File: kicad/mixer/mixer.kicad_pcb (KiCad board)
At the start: 2 copper layers, 100 x 100 mm, 83 parts, among them J1 RETURN_L, J10 CH4_IN, J11 CH5_IN, J12 EURO_PWR_2x5, J2 RETURN_R, J3 SEND_L, J4 SEND_R, J5 MIX_L, J6 MIX_R, J7 CH1_IN, J8 CH2_IN, J9 CH3_IN, U1 TL074, U2 TL074

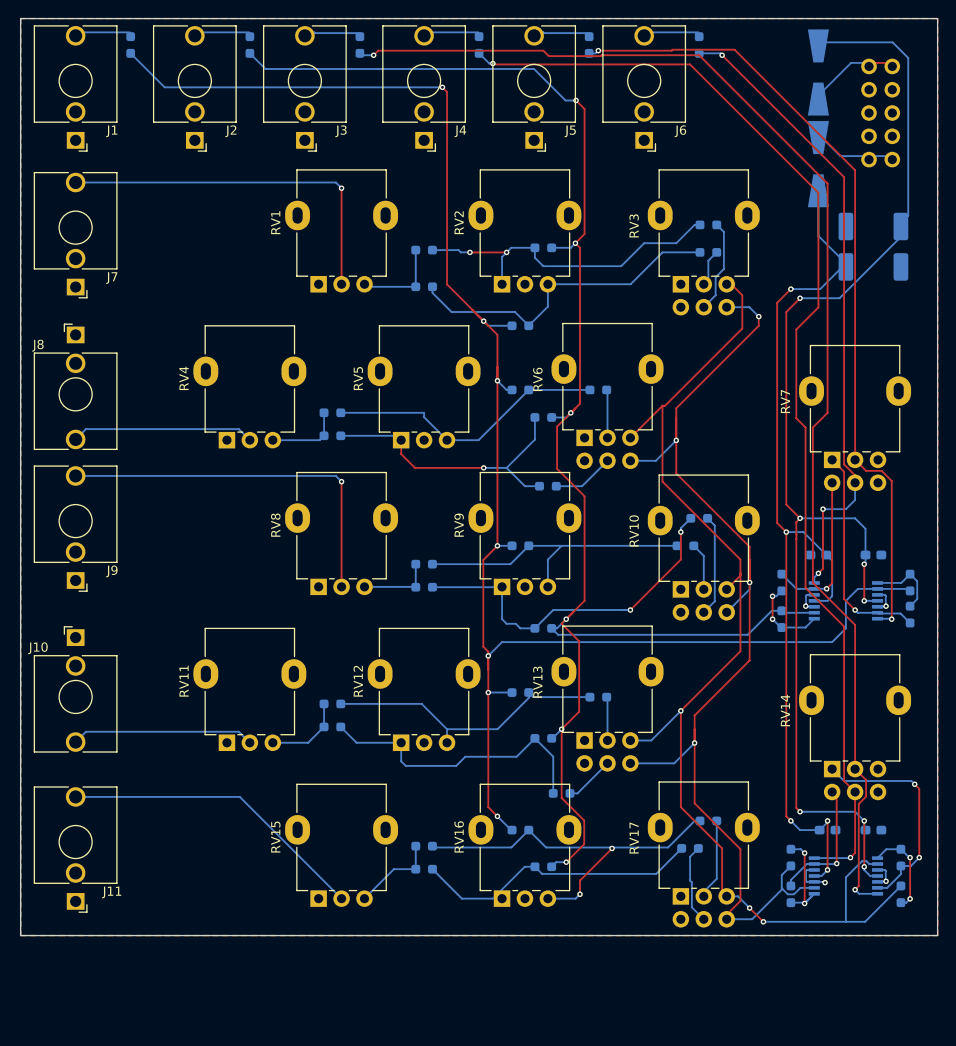
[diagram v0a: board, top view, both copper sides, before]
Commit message: been a minute huh
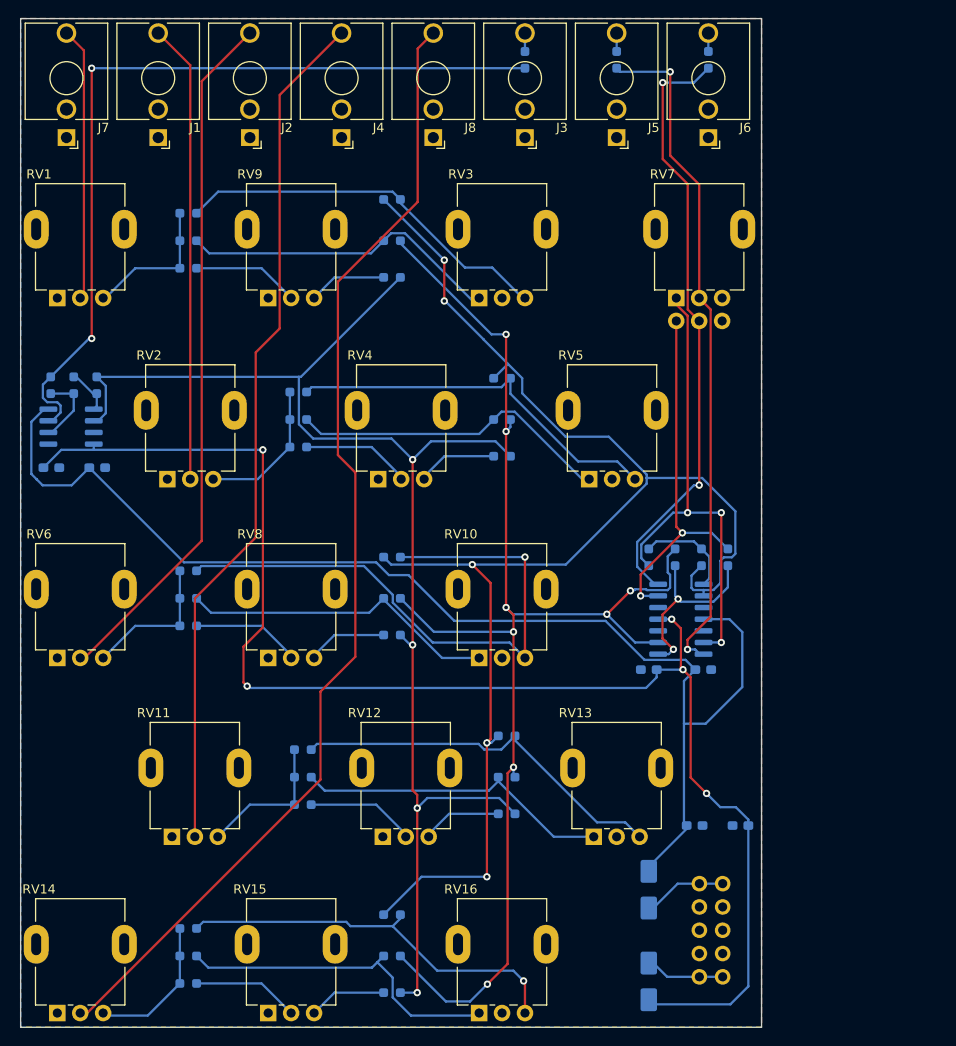
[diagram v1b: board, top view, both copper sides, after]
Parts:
- removed J10: CH4_IN, Connector_Audio:Jack_3.5mm_QingPu_WQP-PJ398SM_Vertical_CircularHoles
- removed J11: CH5_IN, Connector_Audio:Jack_3.5mm_QingPu_WQP-PJ398SM_Vertical_CircularHoles
- removed J9: CH3_IN, Connector_Audio:Jack_3.5mm_QingPu_WQP-PJ398SM_Vertical_CircularHoles
- removed R40, R41: 100k, Resistor_SMD:R_0603_1608Metric_Pad0.98x0.95mm_HandSolder
- removed R42: 10k, Resistor_SMD:R_0603_1608Metric_Pad0.98x0.95mm_HandSolder
- removed R44: 4k7, Resistor_SMD:R_0603_1608Metric_Pad0.98x0.95mm_HandSolder
- removed RV17: A10k, Potentiometer_THT:Potentiometer_Alpha_RD902F-40-00D_Dual_Vertical
- added REF**: LOGO, KitsBlips:logo, B.Cu at (142.0, 56.0)
- C1, C2: footprint Capacitor_SMD:CP_Elec_5x5.3 -> Capacitor_SMD:C_0603_1608Metric_Pad1.08x0.95mm_HandSolder
- D1, D2: value B140-E3/61T -> SS14; footprint Diode_SMD:D_SMA-SMB_Universal_Handsoldering -> Diode_SMD:D_SMA
- J1: value RETURN_L -> MONO_IN; footprint Connector_Audio:Jack_3.5mm_QingPu_WQP-PJ398SM_Vertical_CircularHoles -> KitsBlips:Jack_3.5mm_QingPu_WQP-PJ398SM_Vertical_CircularHoles
- J2: value RETURN_R -> MONO_IN; footprint Connector_Audio:Jack_3.5mm_QingPu_WQP-PJ398SM_Vertical_CircularHoles -> KitsBlips:Jack_3.5mm_QingPu_WQP-PJ398SM_Vertical_CircularHoles
- J3, J5, J6: footprint Connector_Audio:Jack_3.5mm_QingPu_WQP-PJ398SM_Vertical_CircularHoles -> KitsBlips:Jack_3.5mm_QingPu_WQP-PJ398SM_Vertical_CircularHoles
- J4: value SEND_R -> MONO_IN; footprint Connector_Audio:Jack_3.5mm_QingPu_WQP-PJ398SM_Vertical_CircularHoles -> KitsBlips:Jack_3.5mm_QingPu_WQP-PJ398SM_Vertical_CircularHoles
- J7: value CH1_IN -> MONO_IN; footprint Connector_Audio:Jack_3.5mm_QingPu_WQP-PJ398SM_Vertical_CircularHoles -> KitsBlips:Jack_3.5mm_QingPu_WQP-PJ398SM_Vertical_CircularHoles
- J8: value CH2_IN -> MONO_IN; footprint Connector_Audio:Jack_3.5mm_QingPu_WQP-PJ398SM_Vertical_CircularHoles -> KitsBlips:Jack_3.5mm_QingPu_WQP-PJ398SM_Vertical_CircularHoles
- R10, R11, R22, R31, R32, R38: value 10k -> 100k
- R13, R19, R25, R29, R33, R34, R35, R5, R6, R7, R8, R9: value 100k -> 10k
- R3: value 1k -> 10k
- R39: value 4k7 -> 10k
- RV1, RV11, RV15, RV16, RV4, RV5, RV8: footprint Potentiometer_THT:Potentiometer_Alpha_RD901F-40-00D_Single_Vertical -> KitsBlips:Potentiometer_Alpha_RD901F-40-00D_Single_Vertical
- RV10, RV13, RV3: value A10k -> B10k; footprint Potentiometer_THT:Potentiometer_Alpha_RD902F-40-00D_Dual_Vertical -> KitsBlips:Potentiometer_Alpha_RD901F-40-00D_Single_Vertical
- RV12, RV2, RV9: value B10k -> A10k; footprint Potentiometer_THT:Potentiometer_Alpha_RD901F-40-00D_Single_Vertical -> KitsBlips:Potentiometer_Alpha_RD901F-40-00D_Single_Vertical
- RV14, RV6: footprint Potentiometer_THT:Potentiometer_Alpha_RD902F-40-00D_Dual_Vertical -> KitsBlips:Potentiometer_Alpha_RD901F-40-00D_Single_Vertical
- RV7: footprint Potentiometer_THT:Potentiometer_Alpha_RD902F-40-00D_Dual_Vertical -> KitsBlips:Potentiometer_Alpha_RD902F-40-00D_Dual_Vertical
- U1: footprint Package_SO:SSOP-14_5.3x6.2mm_P0.65mm -> Package_SO:SOIC-14_3.9x8.7mm_P1.27mm
- U2: value TL074 -> TL072; footprint Package_SO:SSOP-14_5.3x6.2mm_P0.65mm -> Package_SO:SOIC-8_3.9x4.9mm_P1.27mm
- moved R39 103.9 mm to (105.8, 90.0)
- moved R43 103.8 mm to (108.3, 90.0)
- moved U2 97.7 mm to (105.5, 94.5)
- moved C5 93.4 mm to (108.3, 99.0)
- moved C6 93.4 mm to (103.3, 99.0)
- moved D1 91.0 mm to (168.5, 145.0)
- moved D2 91.0 mm to (168.5, 155.0)
- moved J12 91.0 mm to (175.5, 151.0)
- moved RV14 84.2 mm to (106.5, 150.9), turned to 0 degrees
- moved C1 67.0 mm to (173.5, 138.0), turned to 0 degrees
- moved C2 64.2 mm to (178.5, 138.0), turned to 0 degrees
- moved R3 59.7 mm to (103.3, 90.0)
- moved R35 58.6 mm to (118.3, 152.2)
- moved RV6 57.4 mm to (106.5, 112.2), turned to 0 degrees
- moved R7 56.9 mm to (118.3, 77.2), turned to 180 degrees
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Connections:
- R10 pad 1: Net-(R10-Pad1) -> /controls/SEND
- R11 pad 1: Net-(R11-Pad1) -> /controls/MIX_L
- R11 pad 2: Net-(R10-Pad2) -> Net-(R11-Pad2)
- R12 pad 1: /controls/MIX_L -> /controls/MIX_R
- R12 pad 2: Net-(R11-Pad1) -> Net-(R12-Pad2)
- R13 pad 1: /controls/MIX_L -> Net-(R13-Pad1)
- R14 pad 1: Net-(R14-Pad1) -> /controls/SEND
- R14 pad 2: Net-(R13-Pad2) -> Net-(R14-Pad2)
- R15 pad 1: Net-(R15-Pad1) -> /controls/MIX_L
- R16 pad 2: Net-(R15-Pad1) -> Net-(R13-Pad1)
- R17 pad 1: Net-(R13-Pad2) -> Net-(R17-Pad1)
- R18 pad 1: Net-(R15-Pad1) -> Net-(R18-Pad1)
- R19 pad 2: Net-(R19-Pad2) -> Net-(R17-Pad2)
- R20 pad 1: /controls/MIX_L -> /controls/SEND
- R21 pad 1: Net-(R21-Pad1) -> /controls/MIX_L
- R21 pad 2: Net-(R20-Pad2) -> Net-(R18-Pad1)
- R22 pad 1: Net-(R20-Pad2) -> /controls/MIX_R
- R22 pad 2: Net-(R22-Pad2) -> Net-(R19-Pad1)
- R25 pad 1: /controls/MIX_R -> Net-(R25-Pad1)
- R25 pad 2: Net-(R19-Pad1) -> Net-(R25-Pad2)
- R26 pad 1: Net-(R19-Pad1) -> Net-(R26-Pad1)
- R26 pad 2: Net-(R22-Pad2) -> Net-(R25-Pad2)
- R29 pad 2: Net-(R29-Pad2) -> Net-(R25-Pad2)
- R3 pad 1: Net-(J4-PadT) -> Net-(R3-Pad1)
- R3 pad 2: Net-(R3-Pad2) -> Net-(U2B--)
- R30 pad 1: /controls/MIX_L -> /controls/SEND
- R30 pad 2: Net-(R29-Pad2) -> Net-(R30-Pad2)
- R31 pad 1: Net-(R29-Pad2) -> /controls/MIX_L
- R31 pad 2: Net-(R31-Pad2) -> Net-(R26-Pad1)
- R32 pad 1: Net-(R32-Pad1) -> /controls/MIX_R
- R32 pad 2: Net-(R31-Pad2) -> Net-(R29-Pad1)
- R33 pad 1: Net-(R32-Pad1) -> Net-(R33-Pad1)
- R34 pad 1: /controls/MIX_R -> Net-(R34-Pad1)
- R34 pad 2: Net-(R32-Pad1) -> Net-(R33-Pad2)
- R35 pad 2: Net-(R35-Pad2) -> Net-(R33-Pad2)
- R36 pad 1: /controls/MIX_L -> /controls/SEND
- R36 pad 2: Net-(R35-Pad2) -> Net-(R36-Pad2)
- R37 pad 1: Net-(R37-Pad1) -> /controls/MIX_L
- R37 pad 2: Net-(R37-Pad2) -> Net-(R34-Pad1)
- R38 pad 1: Net-(R35-Pad2) -> /controls/MIX_R
- R38 pad 2: Net-(R38-Pad2) -> Net-(R35-Pad1)
- R4 pad 2: Net-(R4-Pad2) -> Net-(R3-Pad1)
- R43 pad 2: /controls/SEND_L -> /controls/SEND
- R5 pad 1: /controls/MIX_R -> Net-(R5-Pad1)
- R5 pad 2: Net-(J2-PadT) -> Net-(R13-Pad2)
- R6 pad 1: /controls/MIX_L -> Net-(R15-Pad2)
- R6 pad 2: Net-(J1-PadT) -> Net-(R13-Pad2)
- R7 pad 1: Net-(R10-Pad1) -> Net-(R7-Pad1)
- R8 pad 1: /controls/MIX_R -> Net-(R11-Pad2)
- R8 pad 2: Net-(R10-Pad1) -> Net-(R7-Pad2)
- R9 pad 1: Net-(R9-Pad1) -> Net-(R12-Pad2)
- R9 pad 2: Net-(R11-Pad1) -> Net-(R7-Pad2)
- RV1 pad 3: Net-(R10-Pad2) -> Net-(R7-Pad2)
- RV10 pad 1: GND1 -> Net-(R19-Pad1)
- RV10 pad 2: Net-(R21-Pad1) -> GND1
- RV10 pad 3: /controls/SEND_L -> Net-(R18-Pad1)
- RV11 pad 2: Net-(J10-PadT) -> Net-(J4-PadT)
- RV11 pad 3: Net-(R31-Pad2) -> Net-(R25-Pad2)
- RV12 pad 1: Net-(R32-Pad1) -> GND1
- RV12 pad 2: GND1 -> Net-(R25-Pad1)
- RV12 pad 3: Net-(R29-Pad2) -> Net-(R30-Pad2)
- RV13 pad 1: GND1 -> Net-(R29-Pad1)
- RV13 pad 2: Net-(R29-Pad1) -> GND1
- RV13 pad 3: /controls/SEND_L -> Net-(R26-Pad1)
- RV14 pad 1: Net-(U2B--) -> GND1
- RV14 pad 2: Net-(R4-Pad2) -> Net-(J8-PadT)
- RV14 pad 3: unconnected-(RV14-Pad3) -> Net-(R33-Pad2)
- RV15 pad 2: Net-(J11-PadT) -> Net-(R33-Pad1)
- RV15 pad 3: Net-(R38-Pad2) -> Net-(R36-Pad2)
- RV16 pad 1: Net-(R37-Pad1) -> Net-(R35-Pad1)
- RV16 pad 3: Net-(R35-Pad2) -> Net-(R34-Pad1)
- RV2 pad 1: Net-(R10-Pad1) -> GND1
- RV2 pad 2: GND1 -> Net-(J1-PadT)
- RV2 pad 3: Net-(R11-Pad1) -> Net-(R13-Pad2)
- RV3 pad 1: GND1 -> Net-(R12-Pad2)
- RV3 pad 2: Net-(R9-Pad1) -> GND1
- RV3 pad 3: /controls/SEND_L -> Net-(R11-Pad2)
- RV4 pad 2: Net-(J8-PadT) -> Net-(R5-Pad1)
- RV4 pad 3: Net-(R17-Pad2) -> Net-(R14-Pad2)
- RV5 pad 1: Net-(R15-Pad1) -> Net-(R13-Pad1)
- RV5 pad 3: Net-(R13-Pad2) -> Net-(R15-Pad2)
- RV6 pad 2: Net-(R14-Pad1) -> Net-(J2-PadT)
- RV6 pad 3: /controls/SEND_L -> Net-(R17-Pad2)
- RV8 pad 2: Net-(J9-PadT) -> Net-(R17-Pad1)
- RV8 pad 3: Net-(R22-Pad2) -> Net-(R20-Pad2)
- RV9 pad 1: Net-(R19-Pad1) -> GND1
- RV9 pad 2: GND1 -> Net-(R7-Pad1)
- RV9 pad 3: Net-(R20-Pad2) -> Net-(R10-Pad2)
- U2 pad 2: /controls/SEND_L -> /controls/SEND
- U2 pad 4: +12V -> -12V
- U2 pad 7: Net-(R4-Pad2) -> Net-(R3-Pad1)
- U2 pad 8: Net-(R40-Pad1) -> +12V
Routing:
- net /controls/SEND: track 0.00 -> 148.8 mm, vias 0 -> 4
- net Net-(R4-Pad2): track 140.3 -> 0.00 mm, vias 2 -> 0
- net /controls/SEND_L: track 124.7 -> 0.00 mm, vias 3 -> 0
- net Net-(R3-Pad2): track 123.6 -> 0.00 mm, vias 2 -> 0
- net /controls/SEND_R: track 121.1 -> 0.00 mm, vias 4 -> 0
- net Net-(J8-PadT): track 20.0 -> 124.9 mm
- net Net-(R3-Pad1): track 0.00 -> 90.3 mm, vias 0 -> 2
- net Net-(J4-PadT): track 5.91 -> 94.3 mm
- net Net-(J2-PadT): track 5.91 -> 76.1 mm
- net Net-(R18-Pad1): track 0.00 -> 65.3 mm, vias 0 -> 1
- net -12V: track 100.0 -> 158.8 mm
- net Net-(J1-PadT): track 5.91 -> 50.1 mm
- net Net-(R34-Pad1): track 0.00 -> 44.1 mm, vias 0 -> 1
- net Net-(R35-Pad2): track 41.9 -> 0.00 mm, vias 2 -> 0
- net Net-(R11-Pad2): track 0.00 -> 41.9 mm
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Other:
- board size 100 x 100 mm -> 80.8 x 110 mm
- board text added: "JLCJLCJLCJLC"
- board text added: "https://alloyed.me/kb01"
- board text removed: "-12V"
- board text removed: "KEEPOUT"
- board text removed: "shroud"
